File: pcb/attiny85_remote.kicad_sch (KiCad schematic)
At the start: 18 parts, among them IC1 ATTINY85-20MU, J1 RST/DRV, J2 INT/DRV, J3 PWR, Q2 AO3401A, SW1 F2, SW2 F2, SW3 F2, U1 Ai-Thinker-Ra-02

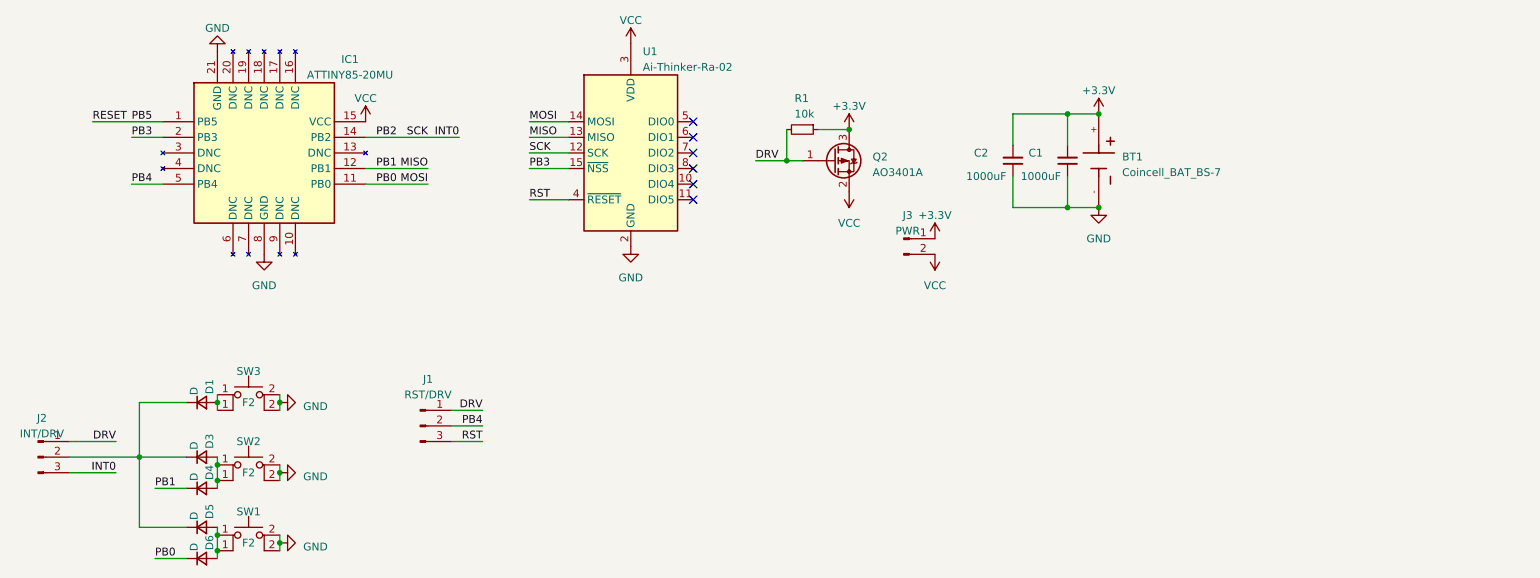
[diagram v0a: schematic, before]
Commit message: gerber out
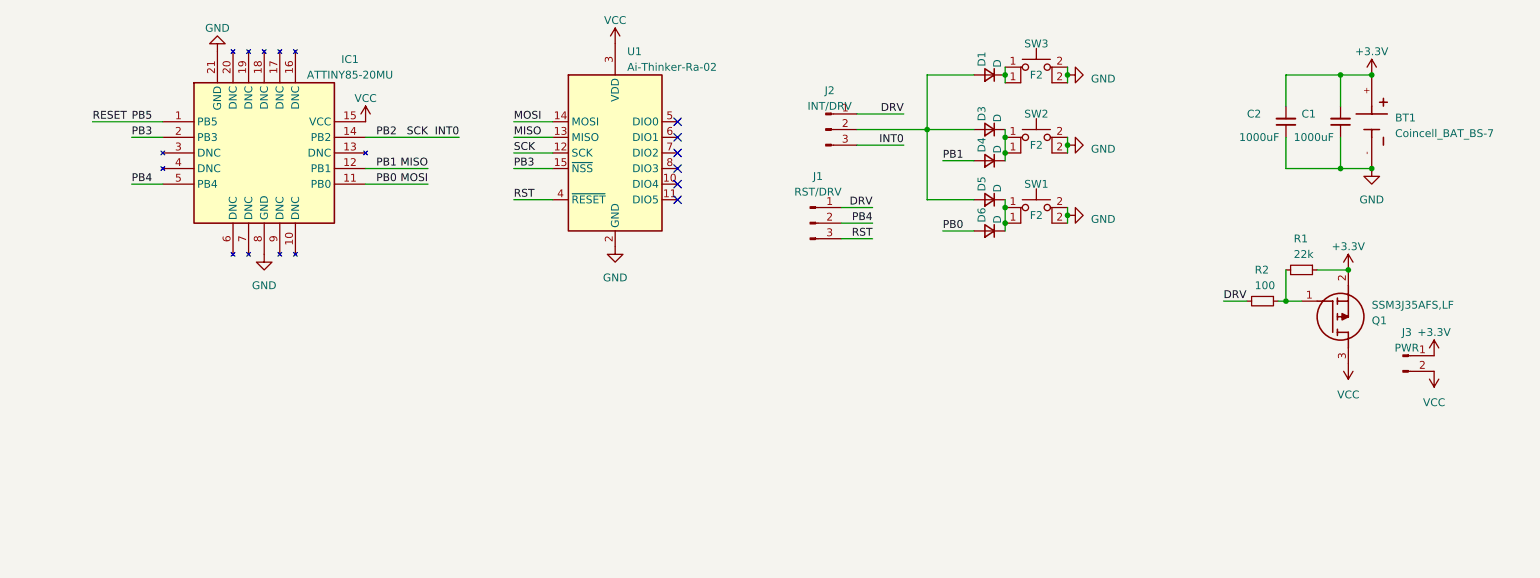
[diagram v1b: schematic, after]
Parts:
- removed Q2: AO3401A, Package_TO_SOT_SMD:SOT-23, symbol Transistor_FET:AO3401A
- added Q1: SSM3J35AFS,LF, Custom:SSM3J35AFSLF, symbol Custom:SSM3J35AFS,LF
- added R2: 100, Resistor_THT:R_Axial_DIN0207_L6.3mm_D2.5mm_P10.16mm_Horizontal, symbol Device:R_Small
- R1: value 10k -> 22k
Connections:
- net +3.3V: now also Q1.2 (S)
- net DRV: now also R2.2; no longer R1.2
- net MISO: now also D4.2 (A); no longer D4.1 (K)
- net MOSI: now also D6.2 (A); no longer D6.1 (K)
- net VCC: now also Q1.3 (D)
- net at SW3.1: now also D1.1 (K); no longer D1.2 (A)
- new net: D1.2 (A), D3.2 (A), D5.2 (A), J2.2 (Pin_2)
- new net: Q1.1 (G), R1.2, R2.1
- new net: D3.1 (K), D4.1 (K), SW2.1
- new net: D5.1 (K), D6.1 (K), SW1.1
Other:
- moved on the sheet: BT1, C1, C2, D1, D3, D4, D5, D6, J1, J2, J3, R1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
